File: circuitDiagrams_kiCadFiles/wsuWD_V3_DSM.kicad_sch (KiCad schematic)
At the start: 46 parts, among them J1 USB_A, J2 Screw Terminal, U1 LD1086D2M33TR, U2 LD1086DT50TR, U3 TCAN332, U4 FT232RL, U5 ATmega644PA-AU, U6 ASDMB-16.000MHz-LC-T, U7 MAX7219, U8 MCP2515-xSO

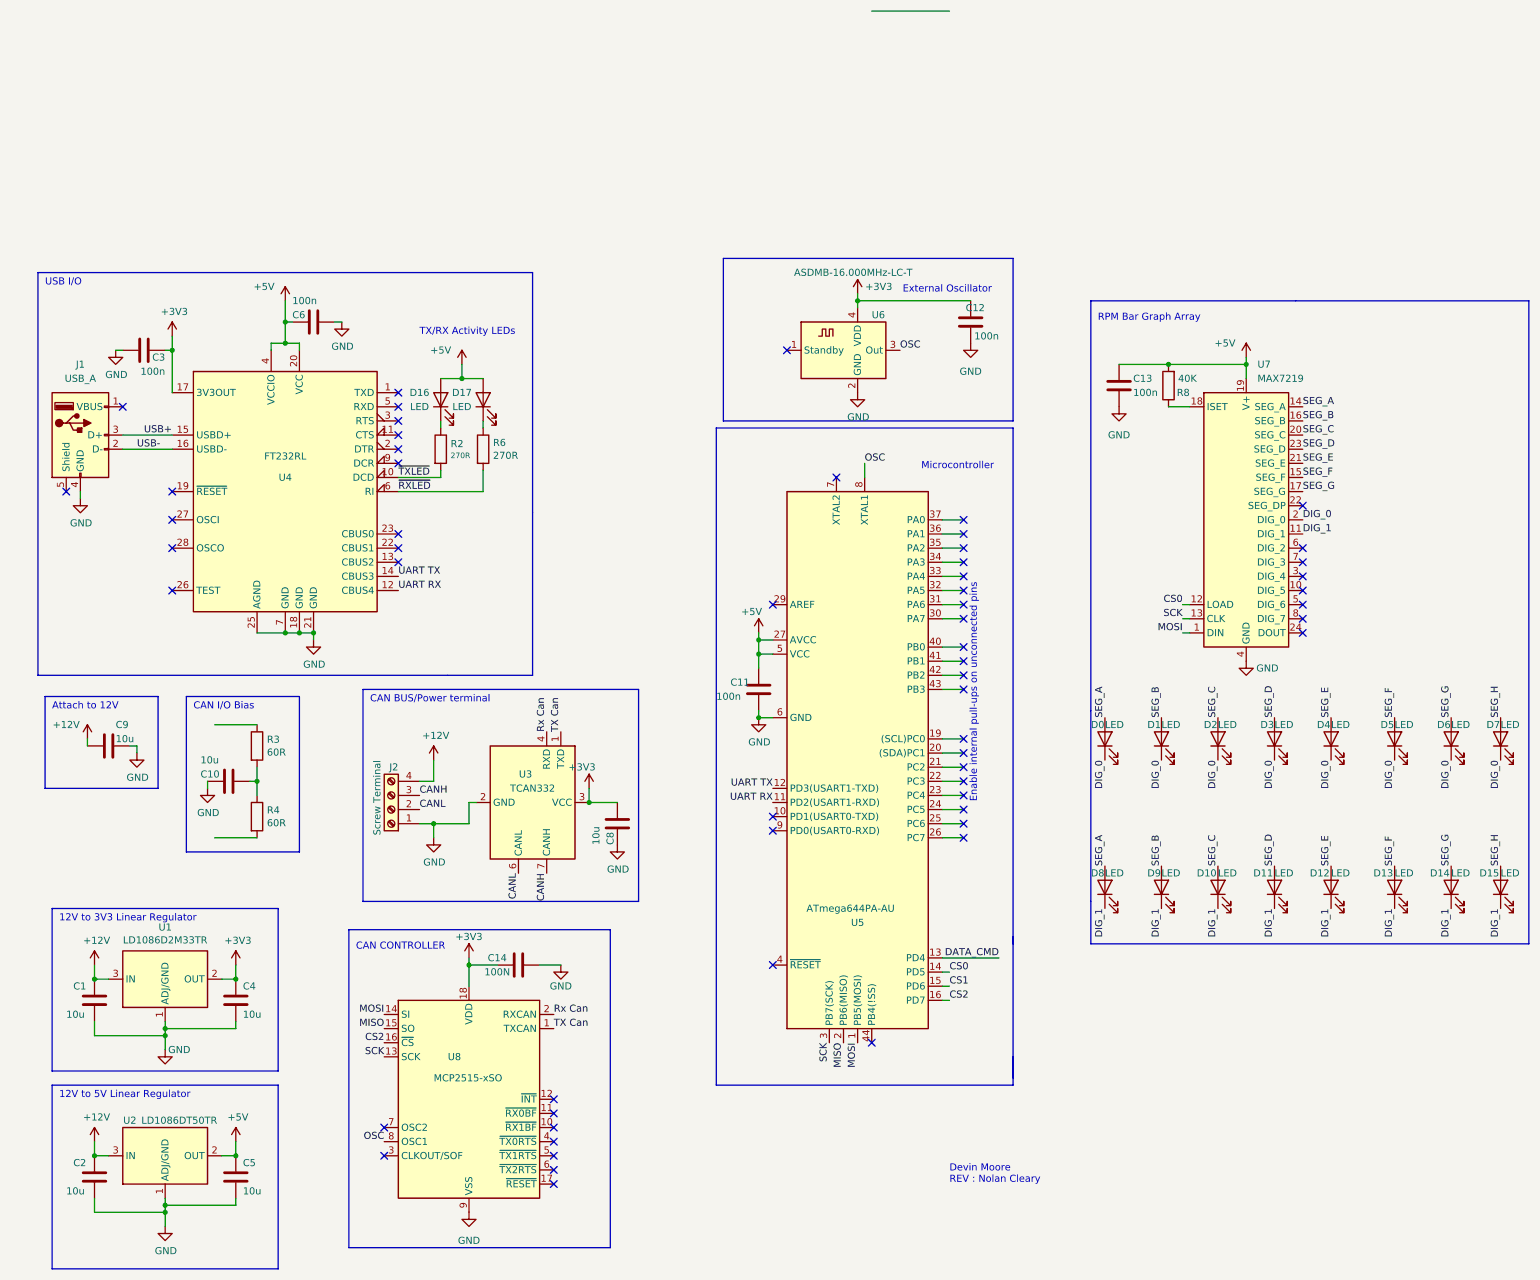
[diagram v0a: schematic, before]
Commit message: Merging older files
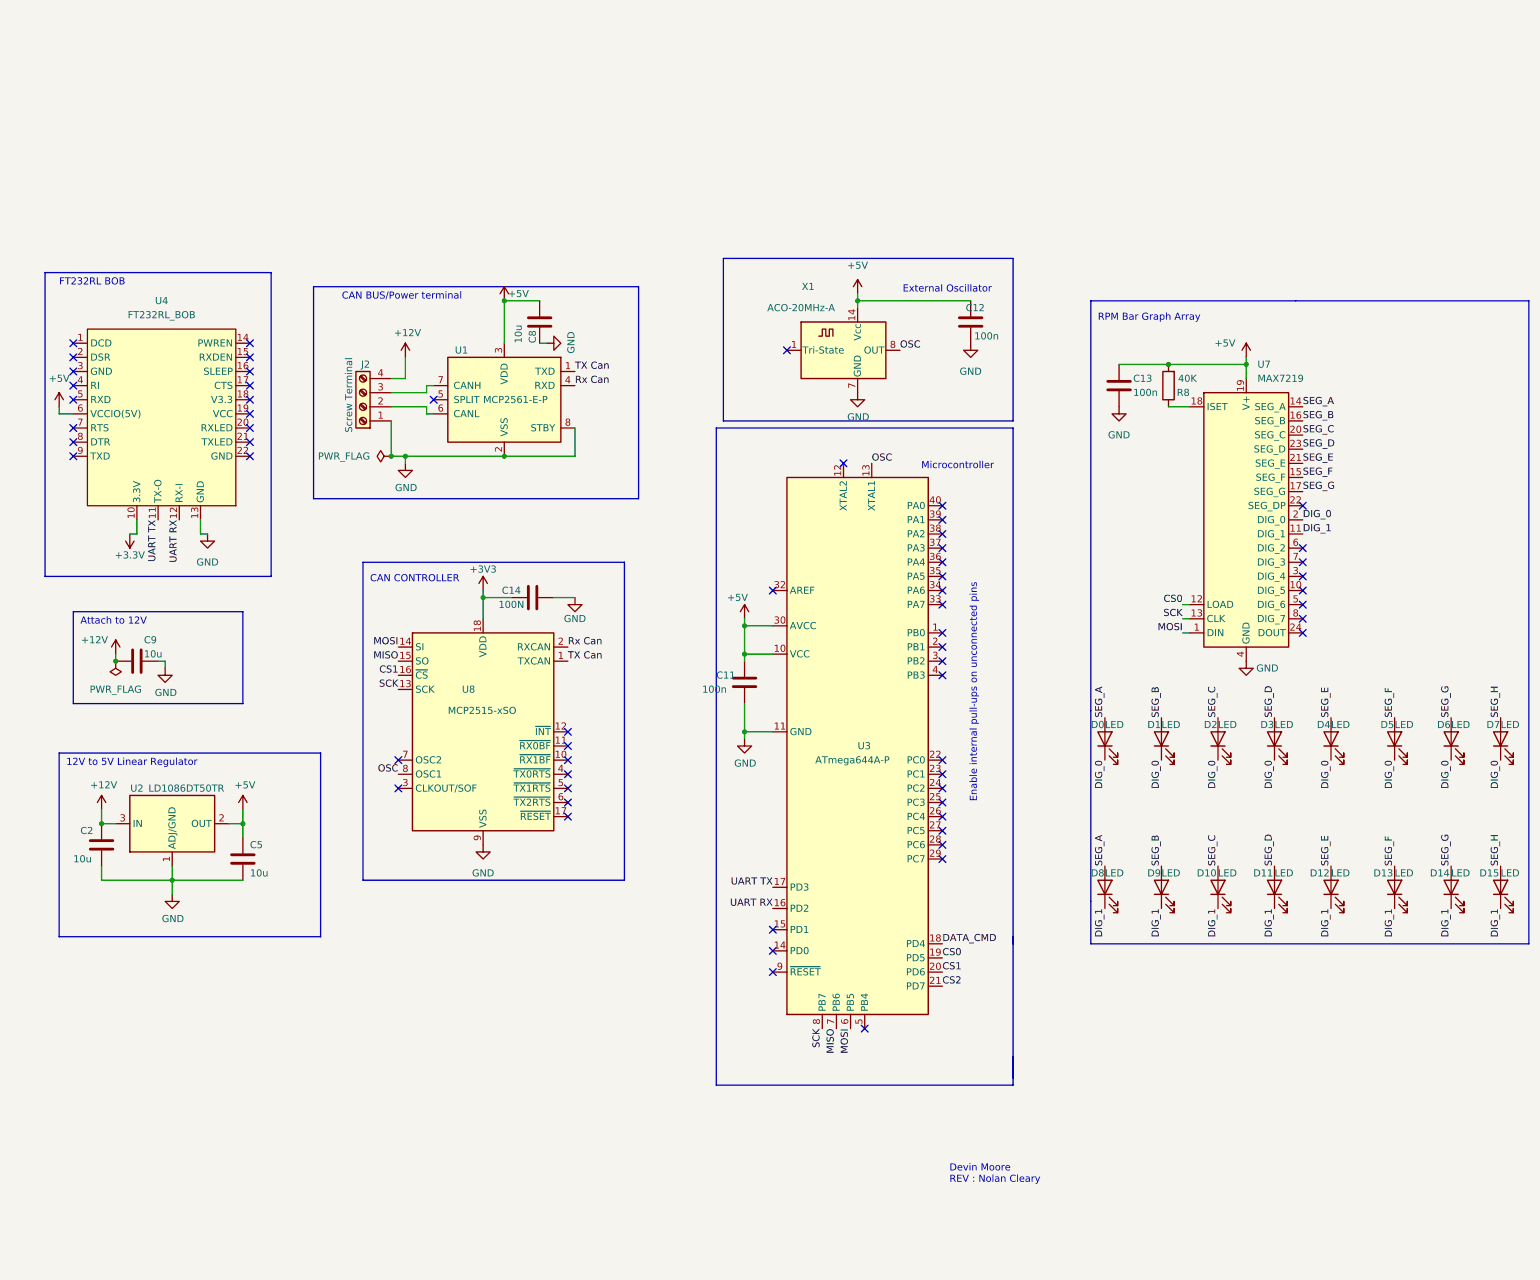
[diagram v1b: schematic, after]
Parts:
- removed C1, C10, C4: 10u, symbol Device:C
- removed C3, C6: 100n, symbol Device:C
- removed D16, D17: LED, symbol Device:LED
- removed J1: USB_A, symbol Connector:USB_A
- removed R2, R6: 270R, symbol Device:R
- removed R3, R4: 60R, symbol Device:R
- removed U1: LD1086D2M33TR, Package_TO_SOT_SMD:TO-263-3_TabPin2, symbol Regulator_Linear:LD1086D2M33TR
- removed U3: TCAN332, symbol Interface_CAN_LIN:TCAN332
- removed U4: FT232RL, Package_SO:SSOP-28_5.3x10.2mm_P0.65mm, symbol Interface_USB:FT232RL
- removed U5: ATmega644PA-AU, Package_QFP:TQFP-44_10x10mm_P0.8mm, symbol MCU_Microchip_ATmega:ATmega644PA-AU
- removed U6: ASDMB-16.000MHz-LC-T, Oscillator:Oscillator_SMD_Abracon_ASDMB-4Pin_2.5x2.0mm, symbol Oscillator:ASDMB-xxxMHz
- added U1: MCP2561-E-P, Package_DIP:DIP-8_W7.62mm, symbol Interface_CAN_LIN:MCP2561-E-P
- added U3: ATmega644A-P, Package_DIP:DIP-40_W15.24mm, symbol MCU_Microchip_ATmega:ATmega644A-P
- added U4: FT232RL_BOB, Connector_PinSocket_2.54mm:PinSocket_1x05_P2.54mm_Vertical, symbol SparkFunBOB:FT232RL_BOB
- added X1: ACO-20MHz-A, Oscillator:Oscillator_DIP-14, symbol Oscillator:ACO-xxxMHz-A
- J2: footprint (none) -> TerminalBlock_4Ucon:TerminalBlock_4Ucon_1x04_P3.50mm_Horizontal
- U7: footprint (none) -> Package_DIP:DIP-24_W7.62mm
- U8: footprint Package_SO:SOIC-18W_7.5x11.6mm_P1.27mm -> Package_DIP:DIP-18_W7.62mm
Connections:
- net +3V3: now also U4.10 (3.3V); no longer C12.2, C8.1
- net +5V: now also C12.2, C8.1, U1.3 (VDD), U3.10 (VCC), U3.30 (AVCC), U4.6 (VCCIO(5V)), X1.14 (Vcc)
- net CS0: now also U3.19 (PD5)
- net CS1: now also U8.16 (~{CS}), U3.20 (PD6)
- net CS2: now also U3.21 (PD7); no longer U8.16 (~{CS})
- net DATA_CMD: now also U3.18 (PD4)
- net GND: now also U1.2 (VSS), U1.8 (STBY), U3.11 (GND), U4.13 (GND), X1.7 (GND)
- net MISO: now also U3.7 (PB6)
- net MOSI: now also U3.6 (PB5)
- net OSC: now also U3.13 (XTAL1), X1.8 (OUT)
- net Rx Can: now also U1.4 (RXD)
- net SCK: now also U3.8 (PB7)
- net TX Can: now also U1.1 (TXD)
- net UART RX: now also U3.16 (PD2), U4.12 (RX-I)
- net UART TX: now also U3.17 (PD3), U4.11 (TX-O)
- net CANH: no longer names the net of J2.3 (Pin_3)
- net CANH: now also U1.7 (CANH)
- net CANL: no longer names the net of J2.2 (Pin_2)
- net CANL: now also U1.6 (CANL)
- no-connect marks 59 -> 62
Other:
- note added: "FT232RL BOB"
- note removed: "12V to 3V3 Linear Regulator"
- note removed: "CAN I/O Bias"
- note removed: "TX/RX Activity LEDs"
- note removed: "USB I/O"
- moved on the sheet: C11, C14, C2, C5, C8, C9, J2, U2, U8

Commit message: Updated schematics
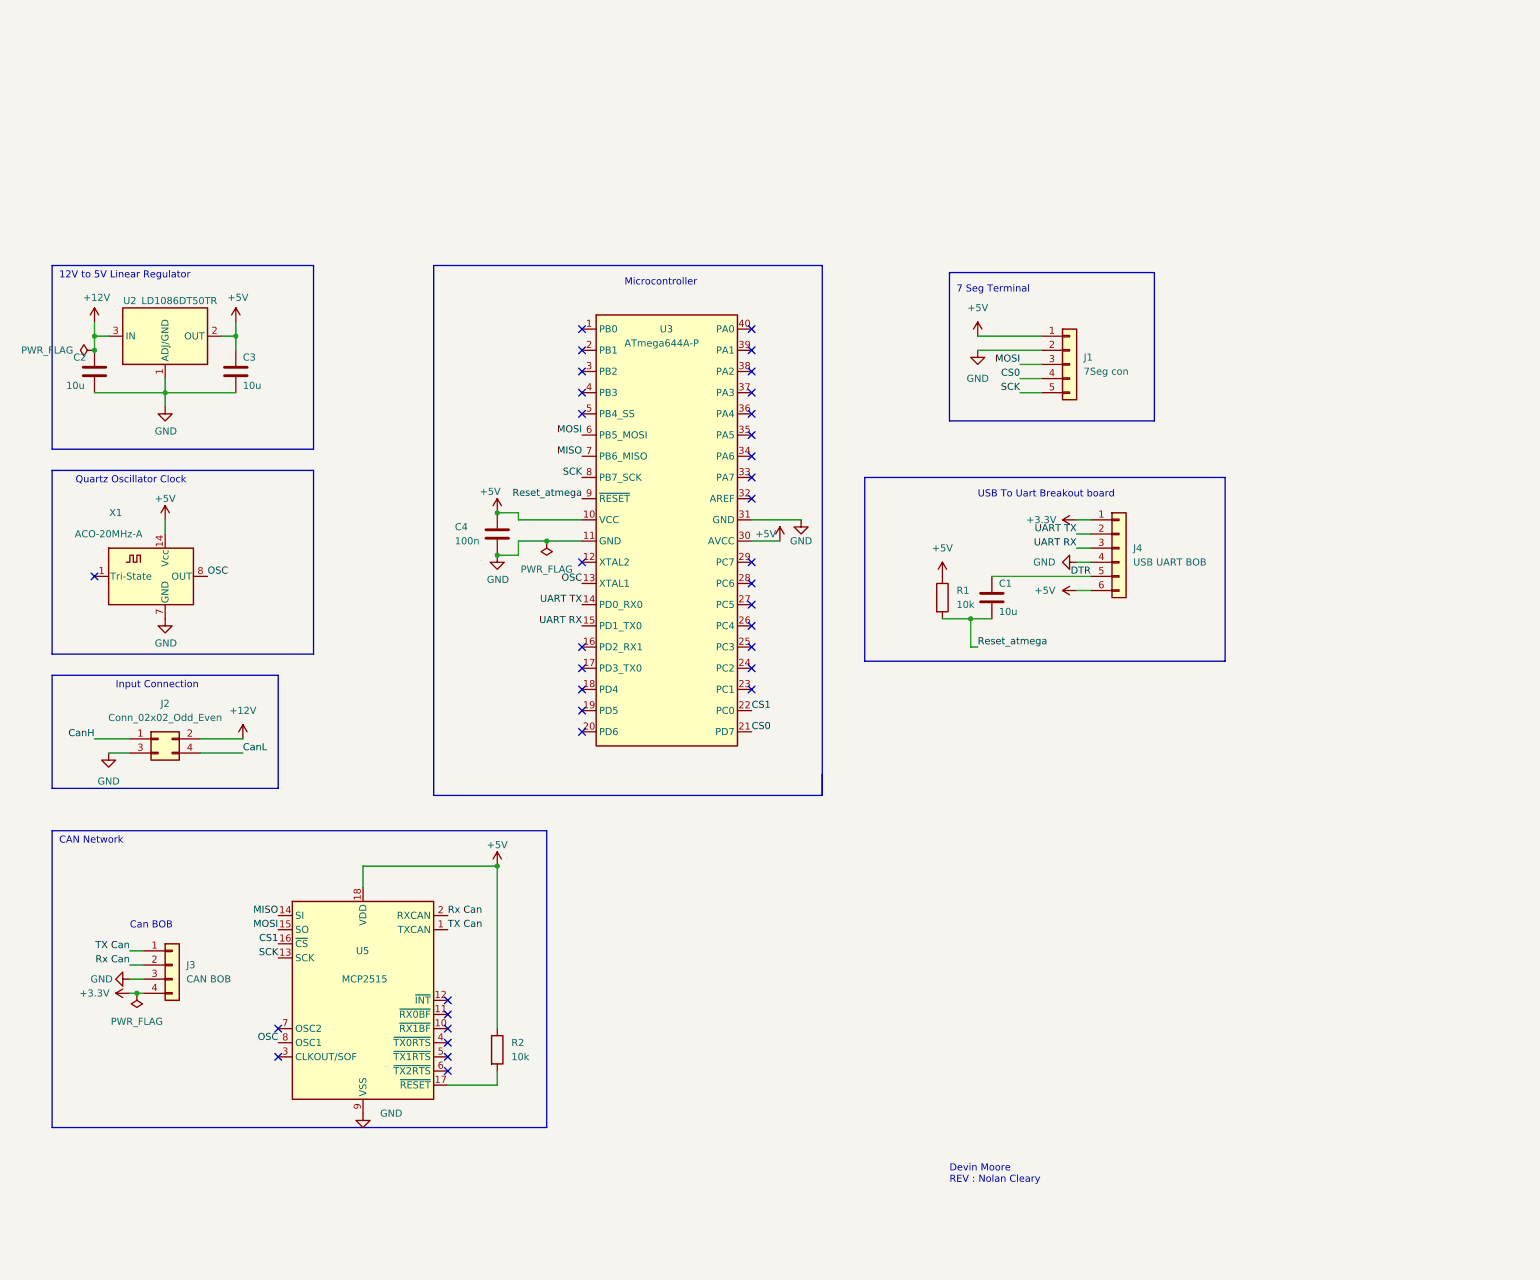
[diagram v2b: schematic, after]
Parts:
- removed C12, C13: 100n, symbol Device:C
- removed C14: 100N, symbol Device:C
- removed C8, C9: 10u, symbol Device:C
- removed D0, D1, D10, D11, D12, D13, D14, D15, D2, D3, D4, D5, D6, D7, D8, D9: LED, symbol Device:LED
- removed J2: Screw Terminal, TerminalBlock_4Ucon:TerminalBlock_4Ucon_1x04_P3.50mm_Horizontal, symbol Connector:Screw_Terminal_01x04
- removed R8: 40K, symbol Device:R
- removed U1: MCP2561-E-P, Package_DIP:DIP-8_W7.62mm, symbol Interface_CAN_LIN:MCP2561-E-P
- removed U4: FT232RL_BOB, Connector_PinSocket_2.54mm:PinSocket_1x05_P2.54mm_Vertical, symbol SparkFunBOB:FT232RL_BOB
- removed U7: MAX7219, Package_DIP:DIP-24_W7.62mm, symbol Driver_LED:MAX7219
- removed U8: MCP2515-xSO, Package_DIP:DIP-18_W7.62mm, symbol Interface_CAN_LIN:MCP2515-xSO
- added C1: 10u, Capacitor_THT:C_Disc_D3.0mm_W1.6mm_P2.50mm, symbol Device:C
- added J1: 7Seg con, Connector_PinSocket_2.00mm:PinSocket_1x05_P2.00mm_Vertical, symbol Connector_Generic:Conn_01x05
- added J2: Conn_02x02_Odd_Even, Connector_PinSocket_2.00mm:PinSocket_2x02_P2.00mm_Vertical, symbol Connector_Generic:Conn_02x02_Odd_Even
- added J3: CAN BOB, Connector_PinHeader_2.00mm:PinHeader_1x04_P2.00mm_Vertical, symbol Connector_Generic:Conn_01x04
- added J4: USB UART BOB, Connector_PinHeader_2.00mm:PinHeader_1x06_P2.00mm_Vertical, symbol Connector_Generic:Conn_01x06
- added R1, R2: 10k, Resistor_THT:R_Axial_DIN0204_L3.6mm_D1.6mm_P5.08mm_Horizontal, symbol Device:R
- added U5: MCP2515, Package_DIP:DIP-18_W7.62mm_Socket, symbol Interface_CAN_LIN:MCP2515-xSO
- C2: footprint (none) -> Capacitor_THT:C_Disc_D3.0mm_W1.6mm_P2.50mm
- C3: renamed from C5; footprint (none) -> Capacitor_THT:C_Disc_D3.0mm_W1.6mm_P2.50mm
- C4: renamed from C11; footprint (none) -> Capacitor_THT:C_Disc_D3.0mm_W1.6mm_P2.50mm
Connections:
- net CS2 is gone; now on net CS0: U3.21 (PD7)
- net +12V: now also J2.2 (Pin_2)
- net +3V3: now also J3.4 (Pin_4), J4.1 (Pin_1)
- net +5V: now also J1.1 (Pin_1), J4.6 (Pin_6), R1.1, R2.1, U5.18 (VDD)
- net CS0: now also J1.4 (Pin_4); no longer U3.19 (PD5)
- net CS1: now also U3.22 (PC0), U5.16 (~{CS}); no longer U3.20 (PD6)
- net GND: now also U3.31 (GND), J1.2 (Pin_2), J2.3 (Pin_3), J3.3 (Pin_3), J4.4 (Pin_4), U5.9 (VSS)
- net MISO: now also U5.14 (SI)
- net MOSI: now also J1.3 (Pin_3), U5.15 (SO)
- net OSC: now also U5.8 (OSC1)
- net Rx Can: now also J3.2 (Pin_2), U5.2 (RXCAN)
- net SCK: now also J1.5 (Pin_5), U5.13 (SCK)
- net TX Can: now also J3.1 (Pin_1), U5.1 (TXCAN)
- net UART RX: now also U3.15 (PD1_TX0), J4.3 (Pin_3); no longer U3.16 (PD2)
- net UART TX: now also U3.14 (PD0_RX0), J4.2 (Pin_2); no longer U3.17 (PD3)
- net Reset_atmega: now reaches U3.9 (~{RESET})
- net Reset_atmega: now also C1.2, R1.2
- net DATA_CMD: no longer names the net of U3.18 (PD4)
- new net: R2.2, U5.17 (~{RESET})
- new net CanH: J2.1 (Pin_1)
- new net CanL: J2.4 (Pin_4)
- new net DTR: C1.1, J4.5 (Pin_5)
- no-connect marks 62 -> 36
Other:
- note added: "7 Seg Terminal"
- note added: "CAN Network"
- note added: "Can BOB"
- note added: "Input Connection"
- note added: "Quartz Oscillator Clock"
- note added: "USB To Uart Breakout board"
- note removed: "Attach to 12V"
- note removed: "CAN BUS/Power terminal"
- note removed: "CAN CONTROLLER"
- note removed: "Enable internal pull-ups on unconnected pins"
- note removed: "External Oscillator"
- note removed: "FT232RL BOB"
- note removed: "RPM Bar Graph Array"
- moved on the sheet: C2, C3, C4, U2, X1
